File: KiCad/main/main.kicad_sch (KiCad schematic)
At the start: 29 parts, among them J1 Hexpansion-Connector, U1 TCA8418, U4 ZD24C64A-XGMT

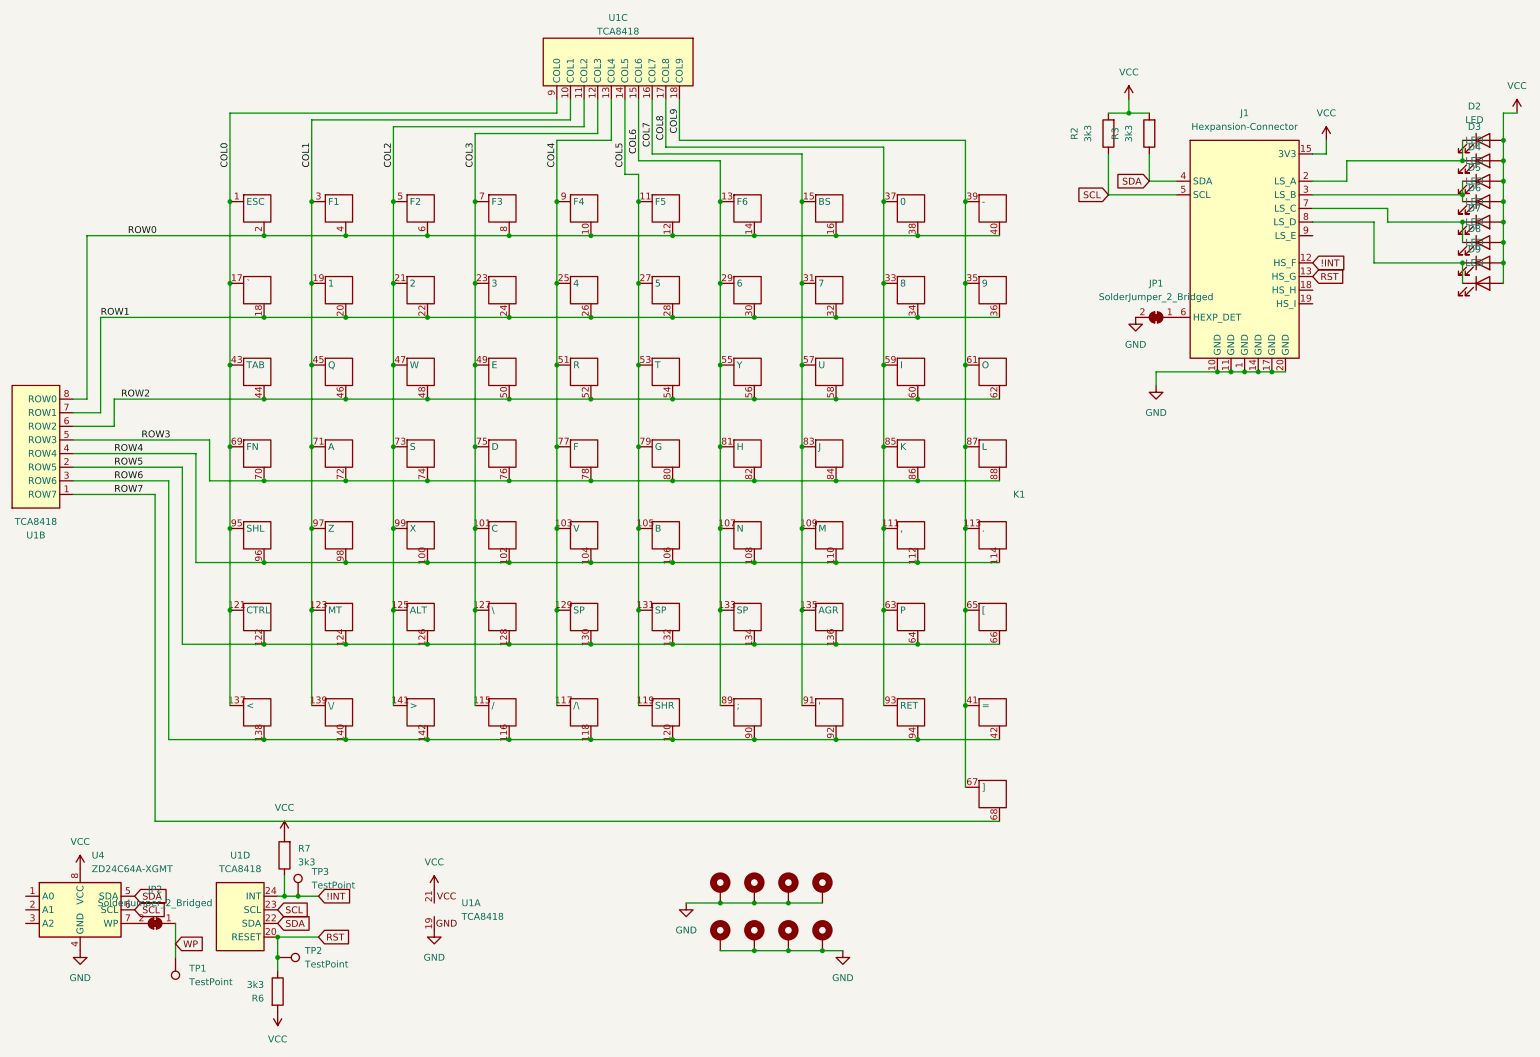
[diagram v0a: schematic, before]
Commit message: Revert "Test App for PWM LED control"
This reverts commit 16f5d63235216fa5ad93ad454a595f19e9ea91df.
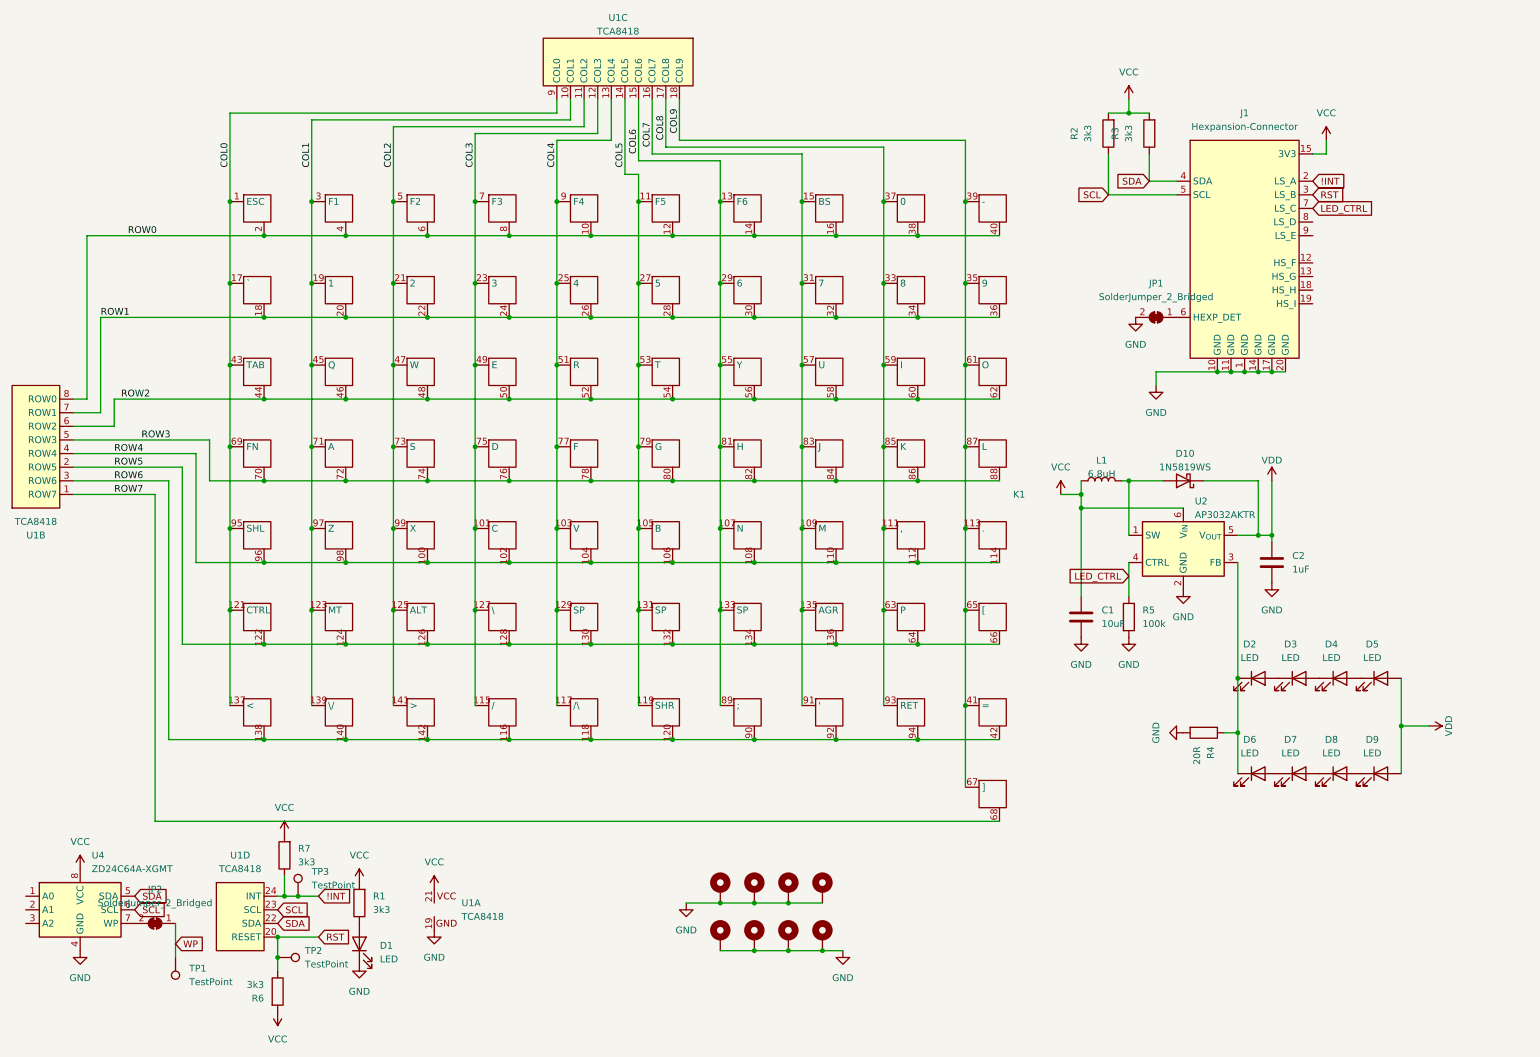
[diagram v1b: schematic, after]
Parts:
- added C1: 10uF, Capacitor_SMD:C_0603_1608Metric_Pad1.08x0.95mm_HandSolder, symbol Device:C
- added C2: 1uF, Capacitor_SMD:C_0603_1608Metric_Pad1.08x0.95mm_HandSolder, symbol Device:C
- added D1: LED, LED_SMD:LED_0603_1608Metric_Pad1.05x0.95mm_HandSolder, symbol Device:LED
- added D10: 1N5819WS, Diode_SMD:D_SOD-323, symbol Diode:1N5819WS
- added L1: 6.8uH, Inductor_SMD:L_0603_1608Metric_Pad1.05x0.95mm_HandSolder, symbol Device:L
- added R1: 3k3, Resistor_SMD:R_0603_1608Metric_Pad0.98x0.95mm_HandSolder, symbol Device:R
- added R4: 20R, Resistor_SMD:R_0603_1608Metric_Pad0.98x0.95mm_HandSolder, symbol Device:R
- added R5: 100k, Resistor_SMD:R_0603_1608Metric_Pad0.98x0.95mm_HandSolder, symbol Device:R
- added U2: AP3032AKTR, Package_TO_SOT_SMD:SOT-23-6, symbol Driver_LED:AP3019AKTR
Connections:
- net !INT: now also J1.2 (LS_A); no longer J1.12 (HS_F)
- net GND: now also C1.2, C2.2, D1.1 (K), R4.2, R5.2, U2.2 (GND)
- net RST: now also J1.3 (LS_B); no longer J1.13 (HS_G)
- net VCC: now also C1.1, L1.1, R1.2, U2.6 (V_{IN}); no longer D2.2 (A), D3.2 (A), D4.2 (A), D5.2 (A), D6.2 (A), D7.2 (A), D8.2 (A), D9.2 (A)
- new net: D1.2 (A), R1.1
- new net: D2.1 (K), D6.1 (K), R4.1, U2.3 (FB)
- new net: D6.2 (A), D7.1 (K)
- new net: D10.2 (A), L1.2, U2.1 (SW)
- new net: D4.2 (A), D5.1 (K)
- new net: D3.2 (A), D4.1 (K)
- new net: D8.2 (A), D9.1 (K)
- new net: D7.2 (A), D8.1 (K)
- new net: D2.2 (A), D3.1 (K)
- new net LED_CTRL: J1.7 (LS_C), R5.1, U2.4 (CTRL)
- new net VDD: C2.1, D10.1 (K), D5.2 (A), D9.2 (A), U2.5 (V_{OUT})
- now unconnected: J1.8 (LS_D)
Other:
- moved on the sheet: D2, D3, D4, D5, D6, D7, D8, D9
